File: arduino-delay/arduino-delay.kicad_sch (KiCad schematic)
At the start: 42 parts, among them J1 Output, J2 CV, J3 Power, J4 Power, J9 Input, SW1 A, SW2 B, SW3 C, U2 TL074

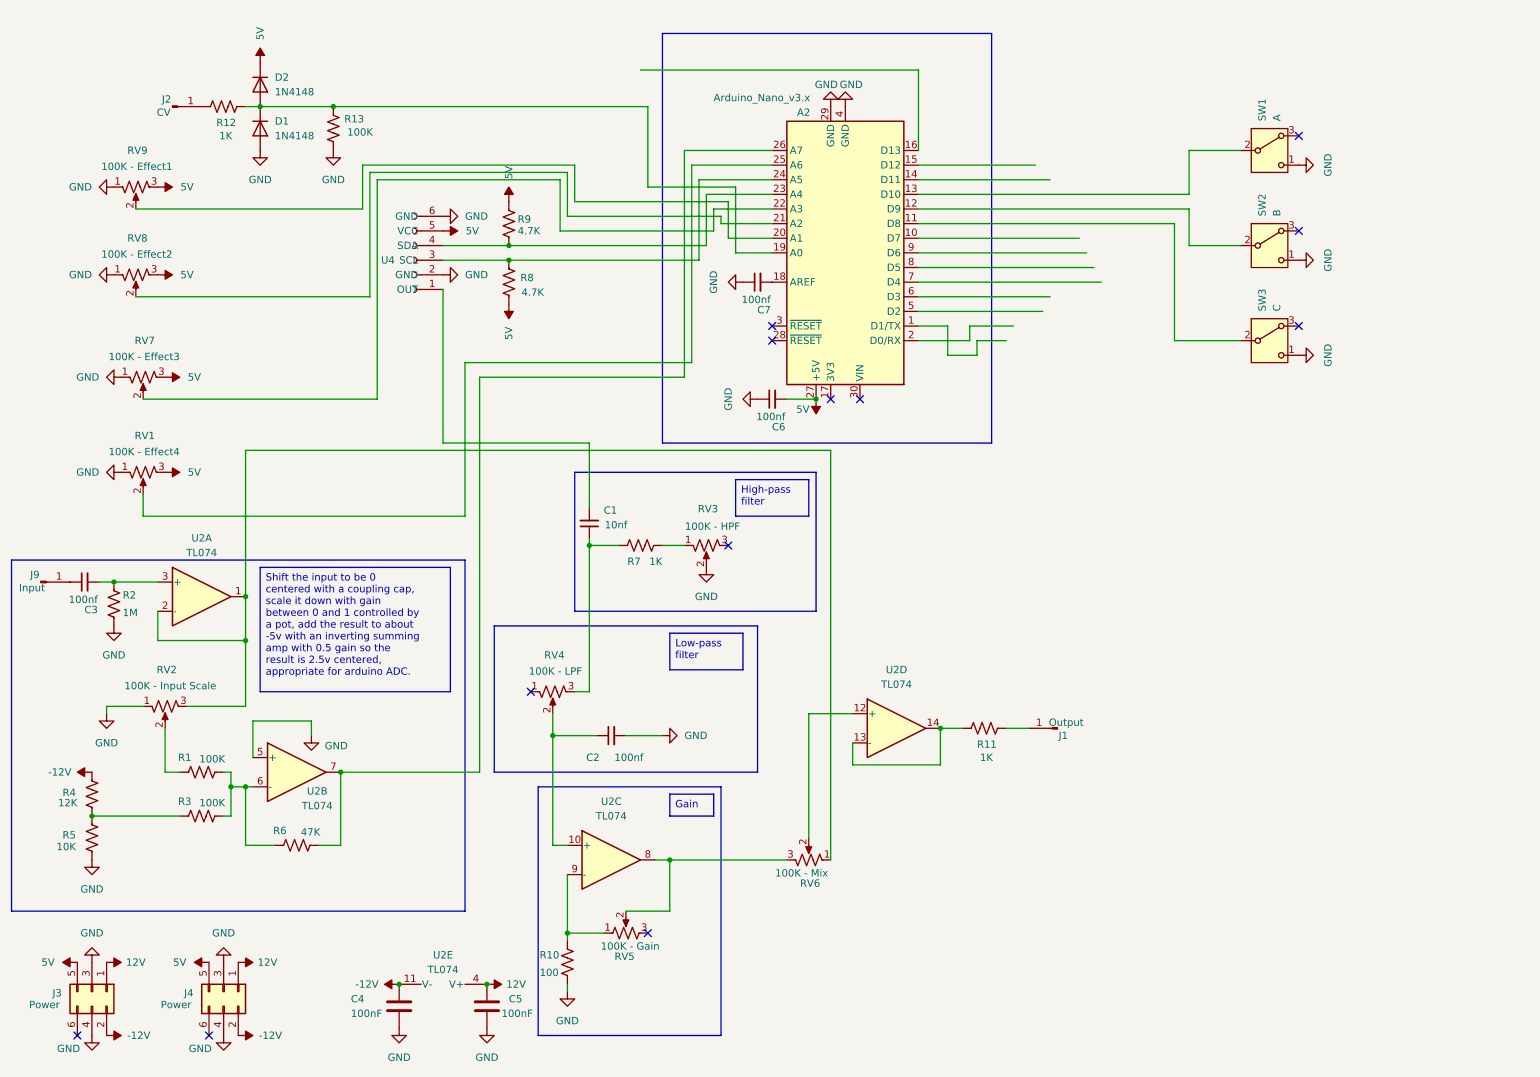
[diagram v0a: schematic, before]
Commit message: Arduino delay progress
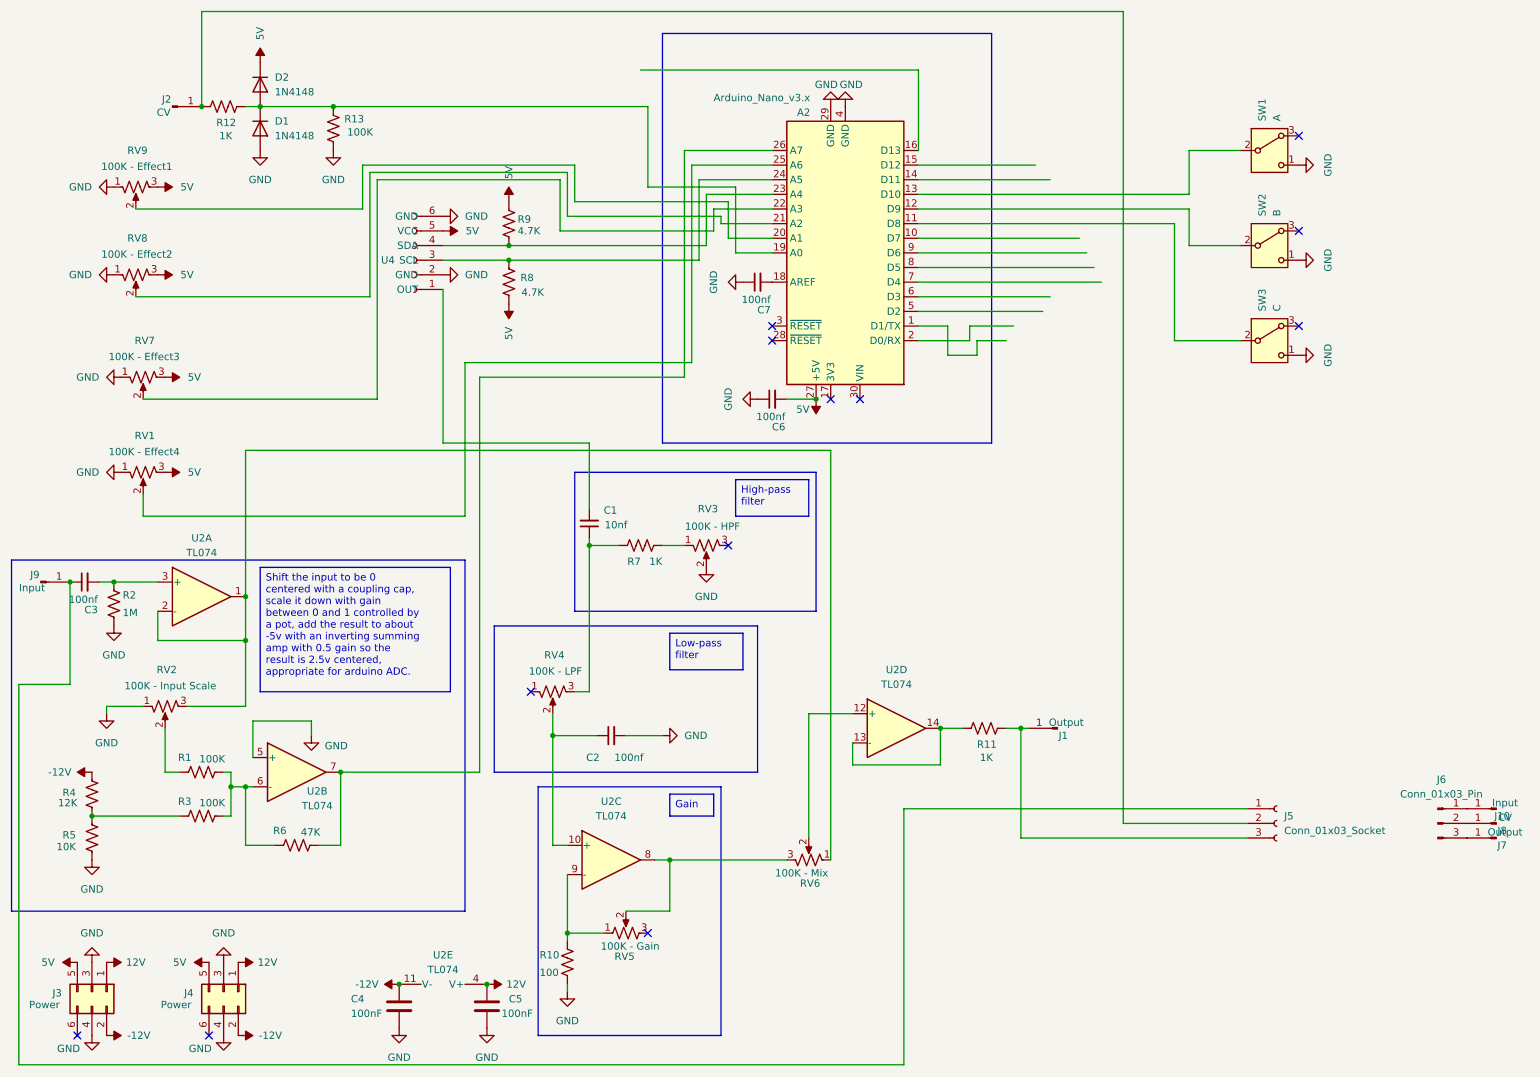
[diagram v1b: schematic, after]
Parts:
- added J10: Input, modular2:banana-jack, symbol Connector:Conn_01x01_Pin
- added J5: Conn_01x03_Socket, Connector_PinSocket_2.54mm:PinSocket_1x03_P2.54mm_Vertical, symbol Connector:Conn_01x03_Socket
- added J6: Conn_01x03_Pin, Connector_PinHeader_2.54mm:PinHeader_1x03_P2.54mm_Vertical, symbol Connector:Conn_01x03_Pin
- added J7: Output, modular2:banana-jack, symbol Connector:Conn_01x01_Pin
- added J8: CV, modular2:banana-jack, symbol Connector:Conn_01x01_Pin
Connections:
- net at C3.1, J9.1 (Pin_1): now also J5.1 (Pin_1)
- net at J2.1 (Pin_1), R12.2: now also J5.2 (Pin_2)
- net at J1.1 (Pin_1), R11.1: now also J5.3 (Pin_3)
- new net: J10.1 (Pin_1), J6.1 (Pin_1)
- new net: J6.2 (Pin_2), J8.1 (Pin_1)
- new net: J6.3 (Pin_3), J7.1 (Pin_1)
